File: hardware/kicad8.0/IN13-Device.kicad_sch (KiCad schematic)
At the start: 17 parts, among them J1 PINHD_1x3_Female, Q2 MMBTA42, T1 Transformer_1P_1S, U1 LM358, U2 STI3508, U3 XIAO-ESP32-C3-DIP

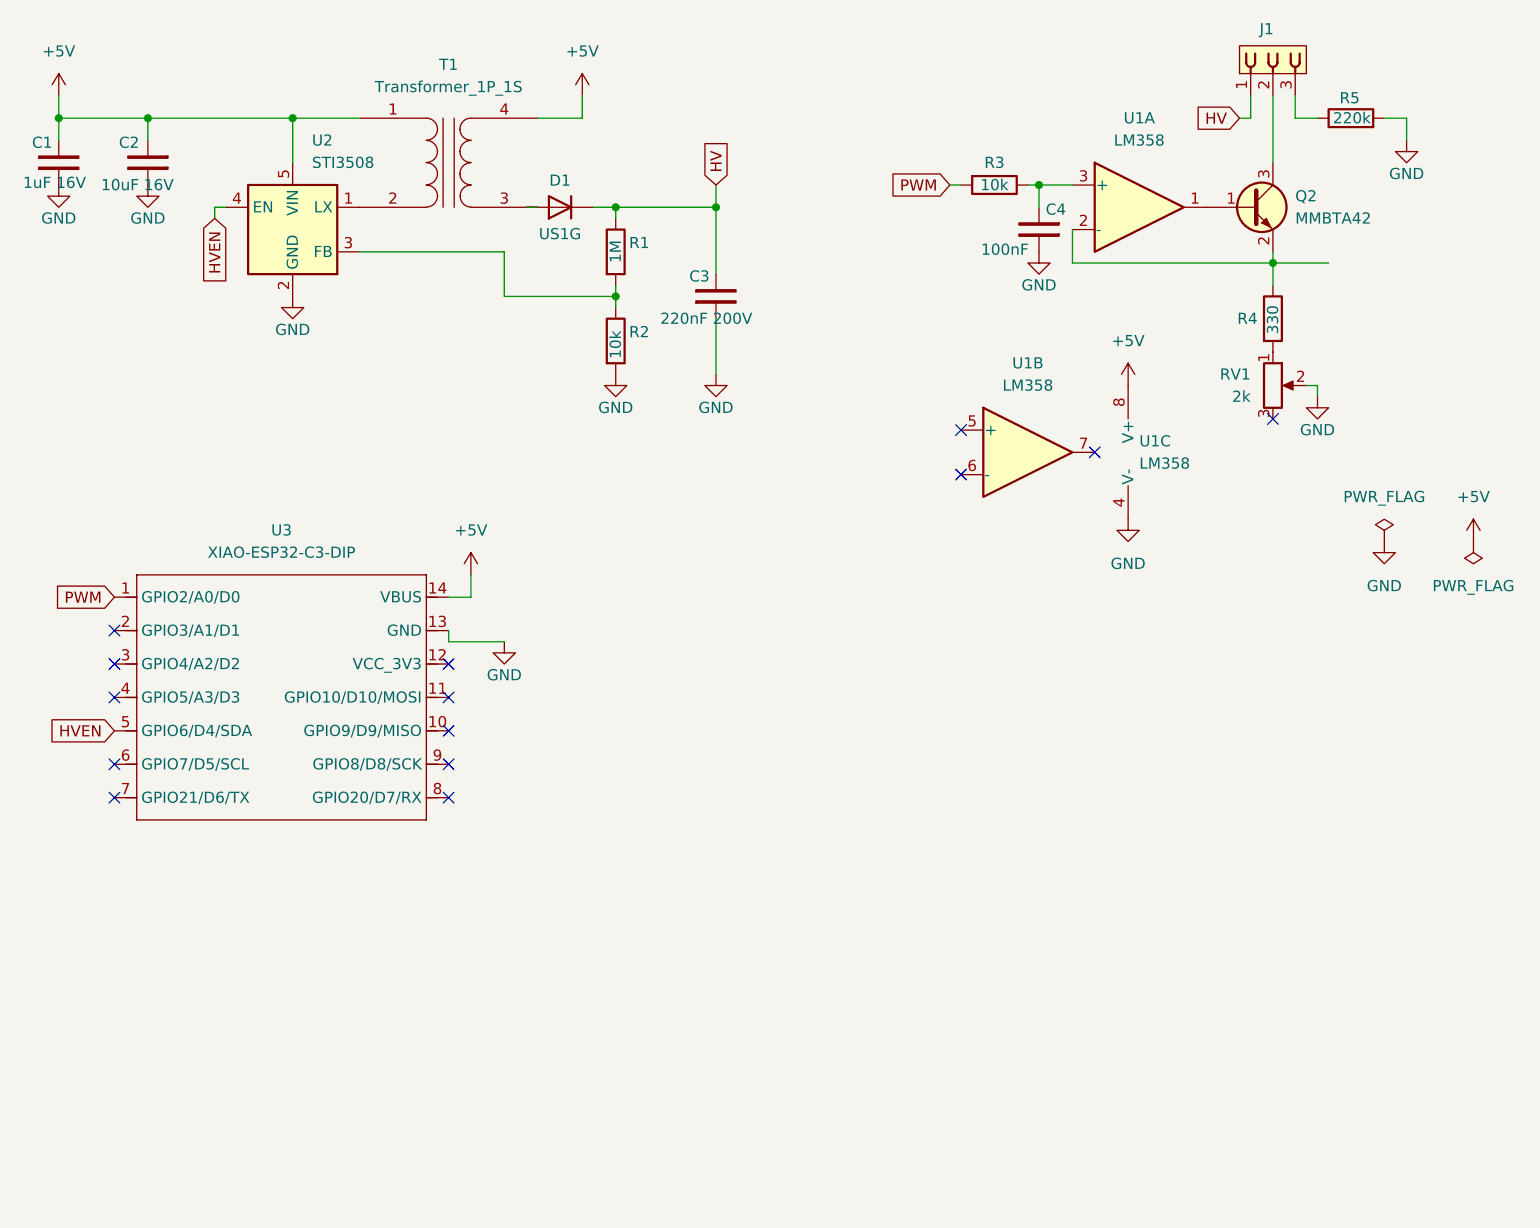
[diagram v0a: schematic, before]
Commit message: esp32c6 module
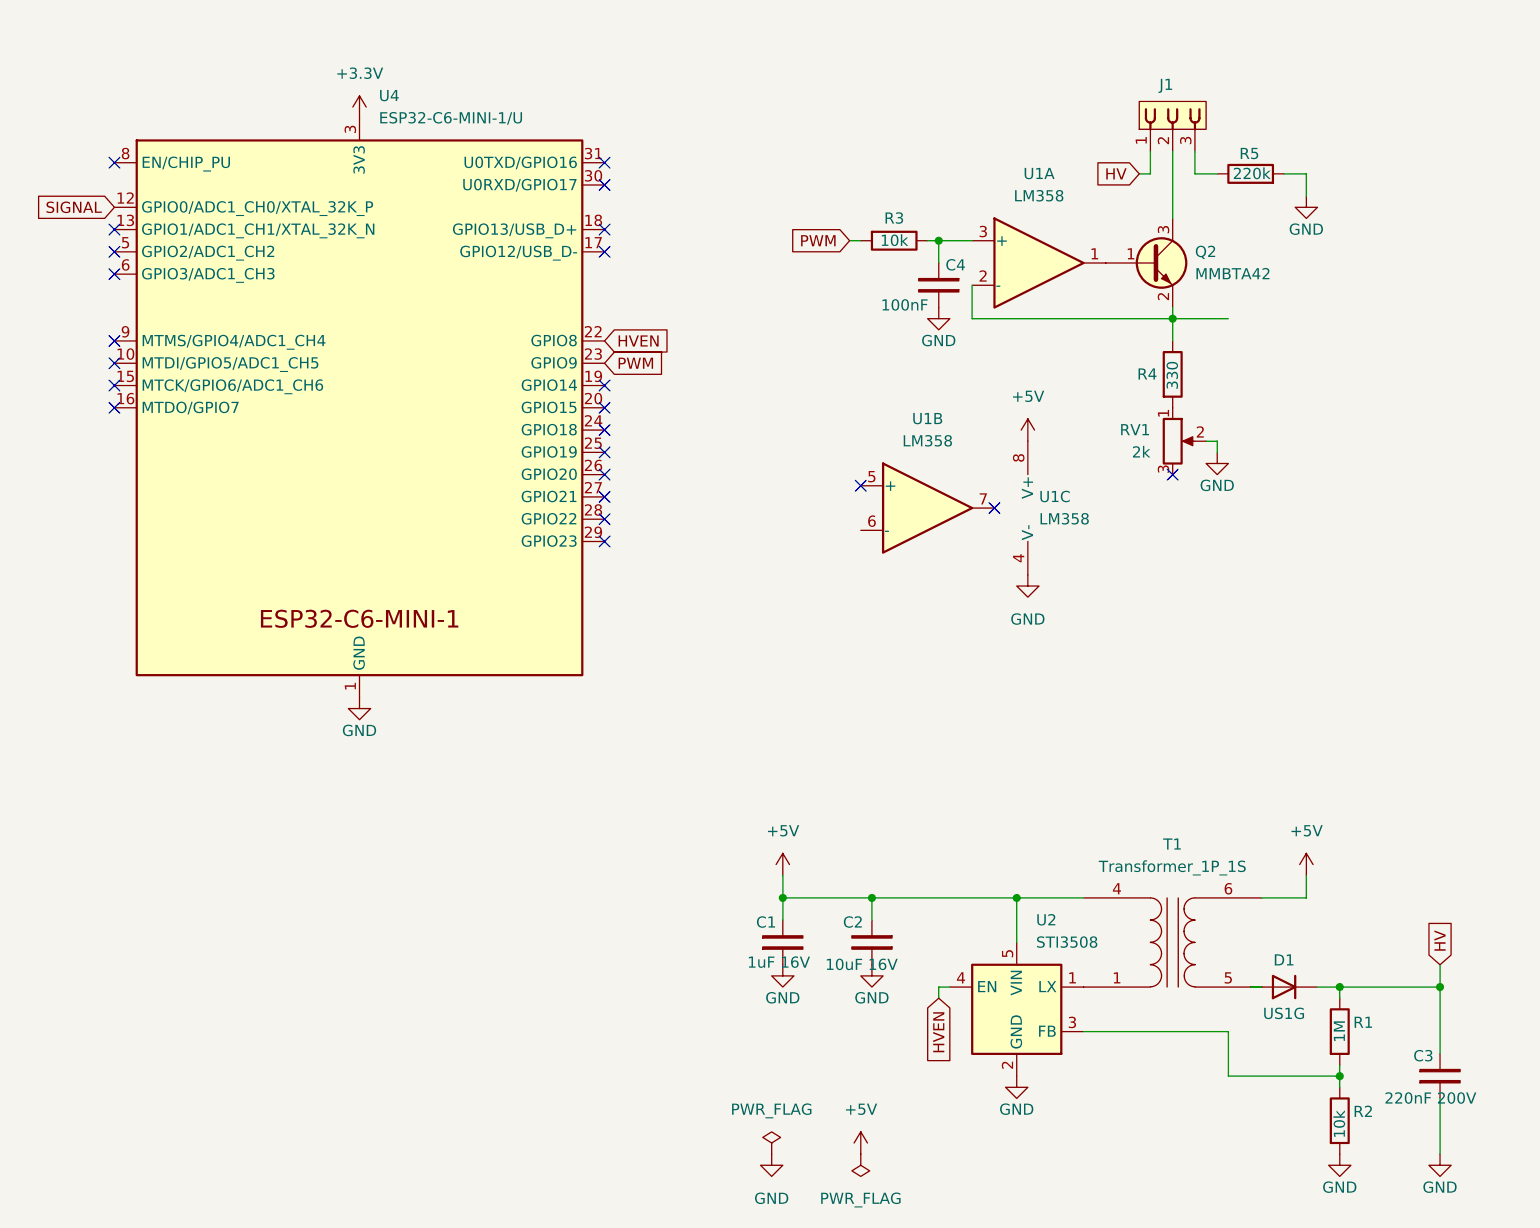
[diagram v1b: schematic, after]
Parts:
- removed U3: XIAO-ESP32-C3-DIP, Module:MOUDLE14P-XIAO-DIP-SMD, symbol Xiao:XIAO-ESP32-C3-DIP
- added U4: ESP32-C6-MINI-1/U, PCM_Espressif:ESP32-C6-MINI-1U, symbol PCM_Espressif:ESP32-C6-MINI-1/U
- T1: footprint (none) -> IN13-Device:EE0504S; symbol Device:Transformer_1P_1S -> IN13-Device:EE0504S_Transformer
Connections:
- net +5V: now also T1.6 (SB); no longer T1.1 (AA)
- net GND: now also U4.1 (GND), U4.11 (GND), U4.14 (GND), U4.2 (GND), U4.36 (GND), U4.37 (GND), U4.38 (GND), U4.39 (GND), U4.40 (GND), U4.41 (GND), U4.42 (GND), U4.43 (GND), U4.44 (GND), U4.45 (GND), U4.46 (GND), U4.47 (GND), U4.48 (GND), U4.49 (GND), U4.50 (GND), U4.51 (GND), U4.52 (GND), U4.53 (GND)
- net HVEN: now also U4.22 (GPIO8)
- net PWM: now also U4.23 (GPIO9)
- net at U2.1 (LX): now also T1.1 (AB); no longer T1.2 (AB)
- net at D1.2 (A): now also T1.5 (SA); no longer T1.3 (SA)
- new net +3.3V: U4.3 (3V3)
- new net SIGNAL: U4.12 (GPIO0/ADC1_CH0/XTAL_32K_P)
- no-connect marks 14 -> 23
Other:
- moved on the sheet: C1, C2, C3, C4, D1, J1, Q2, R1, R2, R3, R4, R5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
